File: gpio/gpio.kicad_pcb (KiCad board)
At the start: 2 copper layers, 96.5 x 66 mm, 20 parts, among them J1 Screw Termial, J2 Screw Terminal, J3 Screw Termial, J4 Screw Termial, J5 I2C, J6 RotaryEncoder, U1 VoltageRegulator, U2 ESP32, U3 TJA1050

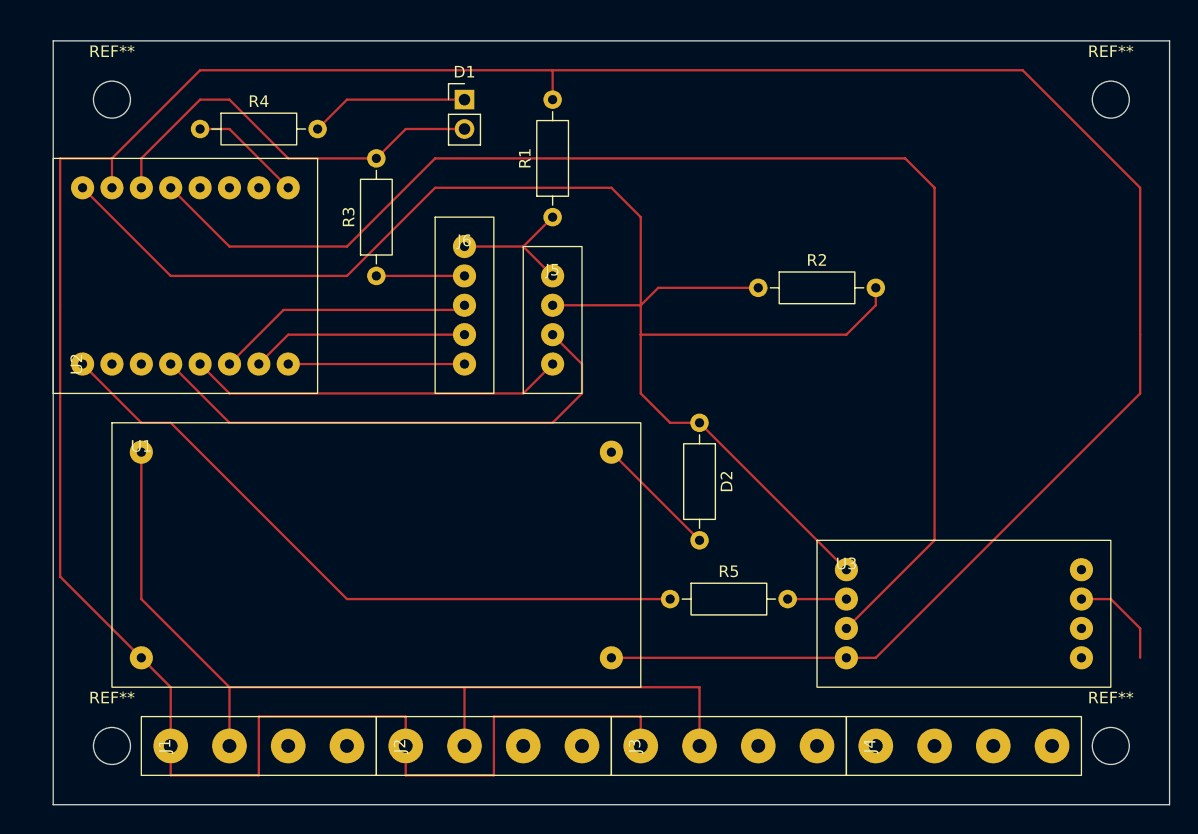
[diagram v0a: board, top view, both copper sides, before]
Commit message: gpio
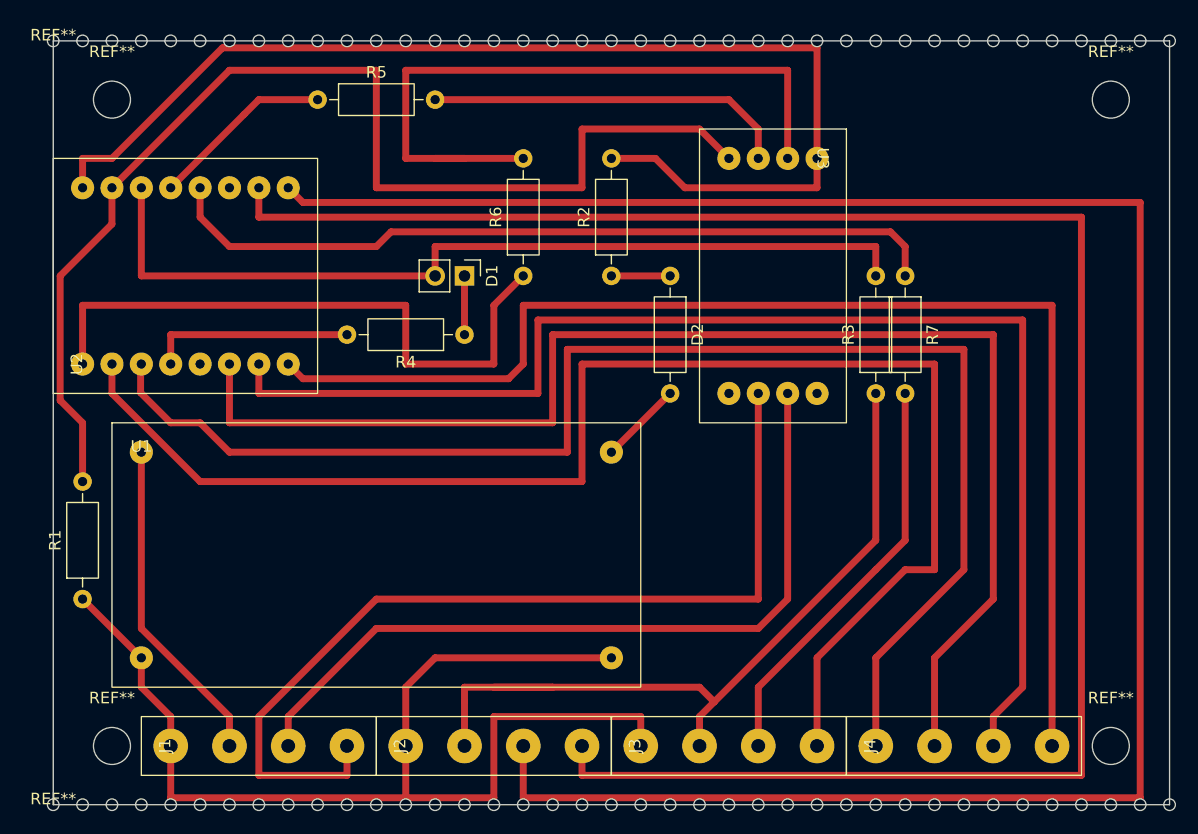
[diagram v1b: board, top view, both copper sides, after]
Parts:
- removed J5: I2C, Peabrain:I2C_Connector
- removed J6: RotaryEncoder, Peabrain:RotaryEncoderConnection
- added R6: ~, Resistor_THT:R_Axial_DIN0207_L6.3mm_D2.5mm_P10.16mm_Horizontal, F.Cu at (66.0, 45.7)
- added R7: ~, Resistor_THT:R_Axial_DIN0207_L6.3mm_D2.5mm_P10.16mm_Horizontal, F.Cu at (99.1, 45.7)
- added REF**: Perforation, Peabrain:Perforation, F.Cu at (25.4, 25.4)
- added REF**: Perforation, Peabrain:Perforation, F.Cu at (25.4, 91.4)
- moved R5 52.9 mm to (48.3, 30.5)
- moved R1 52.4 mm to (27.9, 73.7)
- moved R3 44.4 mm to (96.5, 55.9)
- moved U3 35.7 mm to (91.4, 35.6), turned to -90 degrees
- moved R4 29.0 mm to (61.0, 50.8), turned to 180 degrees
- moved D1 15.2 mm to (61.0, 45.7), turned to -90 degrees
- moved D2 13.0 mm to (78.7, 45.7)
- moved R2 12.7 mm to (73.7, 45.7), turned to 90 degrees
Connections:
- J2 pad 2: /12V -> /3V3
- J2 pad 3: /CANH -> Net-(J2-Pin_3)
- J2 pad 4: /CANL -> Net-(J2-Pin_4)
- J3 pad 2: /12V -> /3V3
- J3 pad 3: /CANH -> Net-(J3-Pin_3)
- J3 pad 4: /CANL -> Net-(J3-Pin_4)
- J4 pad 1: unconnected-(J4-Pin_1-Pad1) -> Net-(J4-Pin_1)
- J4 pad 2: unconnected-(J4-Pin_2-Pad2) -> Net-(J4-Pin_2)
- J4 pad 3: unconnected-(J4-Pin_3-Pad3) -> Net-(J4-Pin_3)
- J4 pad 4: unconnected-(J4-Pin_4-Pad4) -> Net-(J4-Pin_4)
- R4 pad 1: Net-(U2-Pin_9) -> Net-(D1-K)
- R4 pad 2: Net-(D1-K) -> Net-(U2-Pin_4)
- R5 pad 1: Net-(U2-Pin_1) -> Net-(U2-Pin_13)
- R5 pad 2: Net-(U3-Pin_2) -> Net-(U3-Pin_3)
- U2 pad 10: unconnected-(U2-Pin_10-Pad10) -> Net-(J2-Pin_4)
- U2 pad 12: unconnected-(U2-Pin_12-Pad12) -> Net-(U2-Pin_12)
- U2 pad 2: unconnected-(U2-Pin_2-Pad2) -> Net-(J3-Pin_4)
- U2 pad 3: unconnected-(U2-Pin_3-Pad3) -> Net-(J4-Pin_1)
- U2 pad 4: Net-(J5-Pin_3) -> Net-(U2-Pin_4)
- U2 pad 5: Net-(J5-Pin_4) -> unconnected-(U2-Pin_5-Pad5)
- U2 pad 6: Net-(J6-Pin_3) -> Net-(J4-Pin_2)
- U2 pad 7: Net-(J6-Pin_4) -> Net-(J4-Pin_3)
- U2 pad 8: Net-(J6-Pin_5) -> Net-(J4-Pin_4)
- U2 pad 9: Net-(U2-Pin_9) -> Net-(J2-Pin_3)
- U3 pad 3: Net-(U2-Pin_13) -> Net-(U3-Pin_3)
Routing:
- net Net-(J2-Pin_3): track 0.00 -> 183.5 mm
- net Net-(J2-Pin_4): track 0.00 -> 167.6 mm
- net Net-(J3-Pin_4): track 0.00 -> 125.7 mm
- net Net-(J4-Pin_1): track 0.00 -> 122.2 mm
- net Net-(J4-Pin_2): track 0.00 -> 116.4 mm
- net Net-(J4-Pin_3): track 0.00 -> 112.8 mm
- net Net-(J4-Pin_4): track 0.00 -> 110.3 mm
- net /3V3: track 43.4 -> 145.3 mm
- net Net-(U2-Pin_13): track 113.6 -> 15.9 mm
- net /CANL: track 0.00 -> 80.4 mm
- net Net-(U2-Pin_12): track 0.00 -> 68.1 mm
- net /CANH: track 8.67 -> 67.7 mm
- net /GND: track 256.8 -> 200.8 mm
- net Net-(U3-Pin_2): track 5.08 -> 61.0 mm
- net /12V: track 79.4 -> 28.6 mm
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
